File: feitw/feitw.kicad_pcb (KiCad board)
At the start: 2 copper layers, 19.1 x 100 mm, 39 parts, among them J1 Out, J2 Eurorack_Power_10pin_Unshroud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, J3 Trig, Q1 BC847, Q2 BC847, Q3 BC847, U1 TLC555xD, U2 LM358

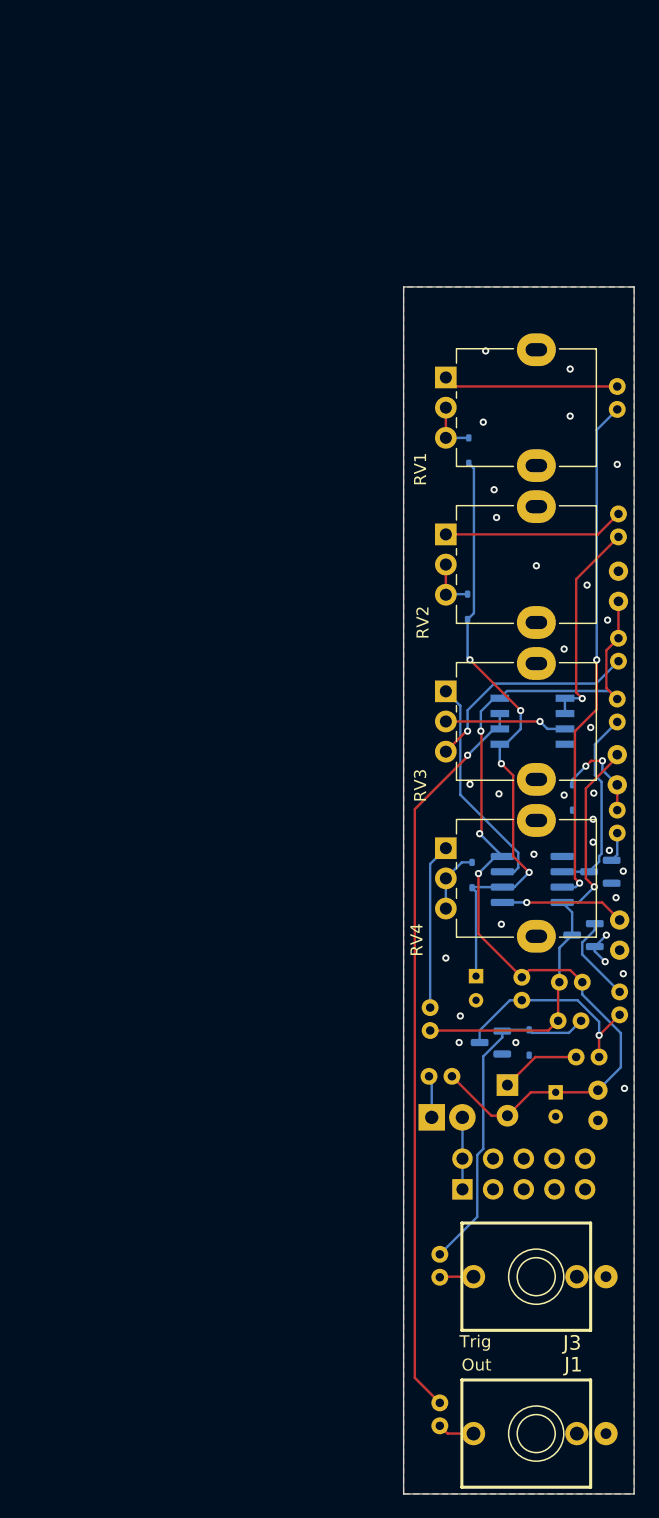
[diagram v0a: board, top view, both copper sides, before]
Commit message: feitw bugfixes
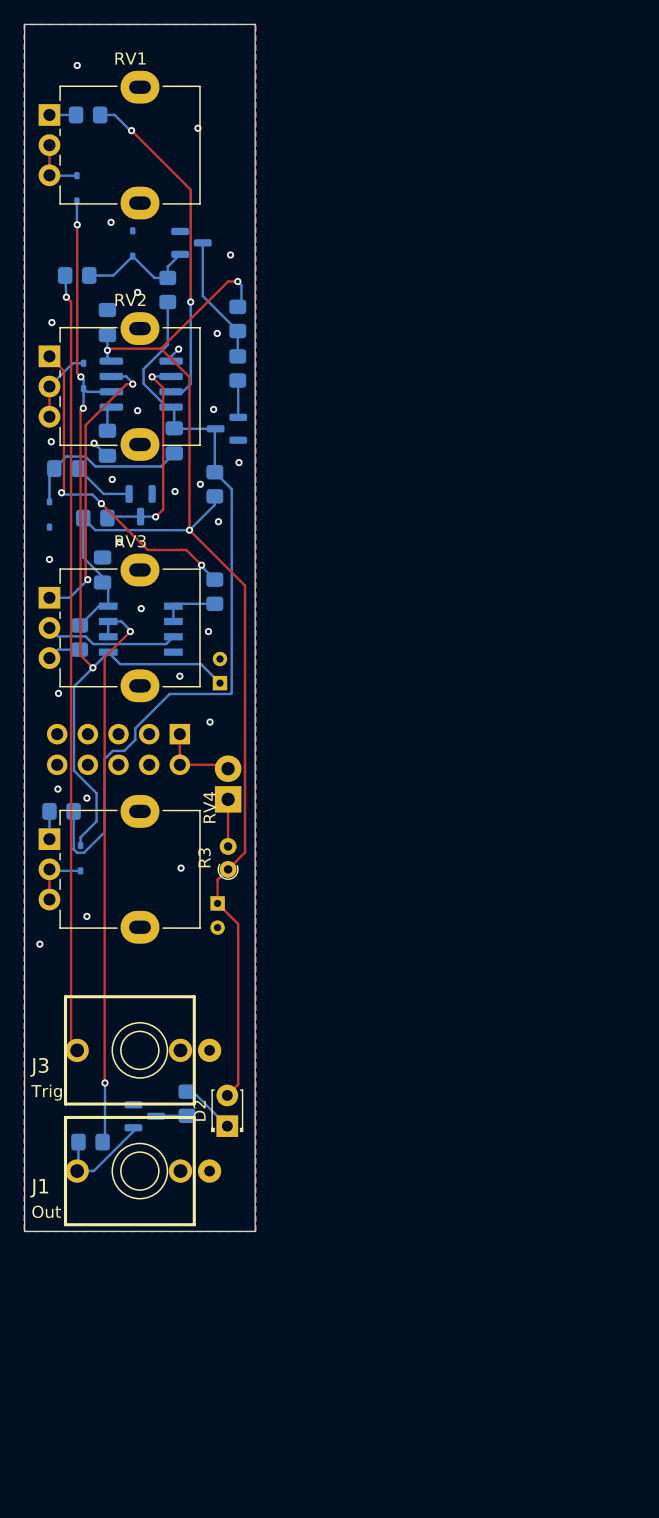
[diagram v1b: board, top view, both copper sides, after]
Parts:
- removed D3: LED, LED_THT:LED_D1.8mm_W3.3mm_H2.4mm
- removed R9: 3k3, Resistor_THT:R_Axial_DIN0204_L3.6mm_D1.6mm_P1.90mm_Vertical
- added D2: LED, LED_THT:LED_D1.8mm_W3.3mm_H2.4mm, F.Cu at (124.4, 139.5)
- added Q4: BC847, Package_TO_SOT_SMD:SOT-23, B.Cu at (117.6, 138.7)
- added R4: 3k3, Resistor_SMD:R_0805_2012Metric_Pad1.20x1.40mm_HandSolder, B.Cu at (121.0, 137.7)
- C1, C4, C5, C7: footprint Capacitor_THT:C_Disc_D3.0mm_W1.6mm_P2.50mm -> Capacitor_SMD:C_0805_2012Metric_Pad1.18x1.45mm_HandSolder
- R1, R10, R11, R12, R13, R14, R15, R2, R5, R6, R7, R8: footprint Resistor_THT:R_Axial_DIN0204_L3.6mm_D1.6mm_P1.90mm_Vertical -> Resistor_SMD:R_0805_2012Metric_Pad1.20x1.40mm_HandSolder
- R3: moved to F.Cu
- moved R10 88.3 mm to (112.0, 69.0), turned to 0 degrees
- moved D4 73.9 mm to (116.6, 66.4), turned to 90 degrees
- moved Q3 70.7 mm to (121.4, 66.3), turned to 0 degrees
- moved R11 69.6 mm to (119.5, 70.2), turned to -90 degrees
- moved R7 62.2 mm to (125.3, 76.8), turned to -90 degrees
- moved C7 61.3 mm to (114.1, 93.5), turned to -90 degrees
- moved R8 59.4 mm to (125.3, 72.7)
- moved C4 58.0 mm to (114.5, 83.0)
- moved R5 54.7 mm to (111.1, 85.0), turned to 180 degrees
- moved U1 52.3 mm to (117.3, 78.0)
- moved Q2 51.3 mm to (124.4, 81.8)
- moved R6 51.3 mm to (123.4, 86.3), turned to 90 degrees
- moved R1 50.2 mm to (112.9, 55.8), turned to 180 degrees
- moved D5 49.3 mm to (109.7, 88.8)
- moved Q1 48.7 mm to (117.2, 88.1), turned to -90 degrees
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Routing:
- net Net-(J3-PadT): track 2.81 -> 64.7 mm, vias 0 -> 1
- net +12V: track 78.2 -> 108.8 mm
- net Net-(Q2-C): track 37.1 -> 64.4 mm, vias 1 -> 0
- net Net-(D6-K): track 51.0 -> 71.2 mm
- net Net-(D4-K): track 27.7 -> 10.3 mm
- net Net-(R15-Pad1): track 18.4 -> 2.79 mm, vias 1 -> 0
- net Net-(U1-Q): track 42.4 -> 28.3 mm
- net Net-(U2B--): track 61.2 -> 47.3 mm, vias 1 -> 2
- net Net-(R13-Pad2): track 15.0 -> 28.2 mm, vias 0 -> 3
- net Net-(U2A--): track 17.8 -> 4.78 mm, vias 1 -> 0
- net Net-(R1-Pad2): track 14.5 -> 2.20 mm
- net Net-(R14-Pad2): track 13.7 -> 2.30 mm
- net Net-(U1-CV): track 10.3 -> 2.09 mm, vias 1 -> 0
- net Net-(Q3-C): track 18.0 -> 10.6 mm, vias 1 -> 0
- net Net-(D3-K): track 6.66 -> 0.00 mm
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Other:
- board text removed: "Clandestine Circutry"
